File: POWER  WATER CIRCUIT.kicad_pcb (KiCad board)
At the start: 2 copper layers, 88.8 x 71.8 mm, 84 parts, among them IC1 DW01, J2 IN-, J3 IN+, J5 OUT +, J6 OUT -, Q1 FS8205A, Q2 BC817, Q3 IRLML5203, Q4 BC817, Q5 BC817, Q6 BC817, SW1 SW_MEC_5G, SW2 SW_MEC_5G, U1 LM2596S-ADJ, U2 TP4056, U3 LM1117MP-3.3, U4 ESP32-WROOM-32, U5 SIM800L-CORE, U6 MT3608

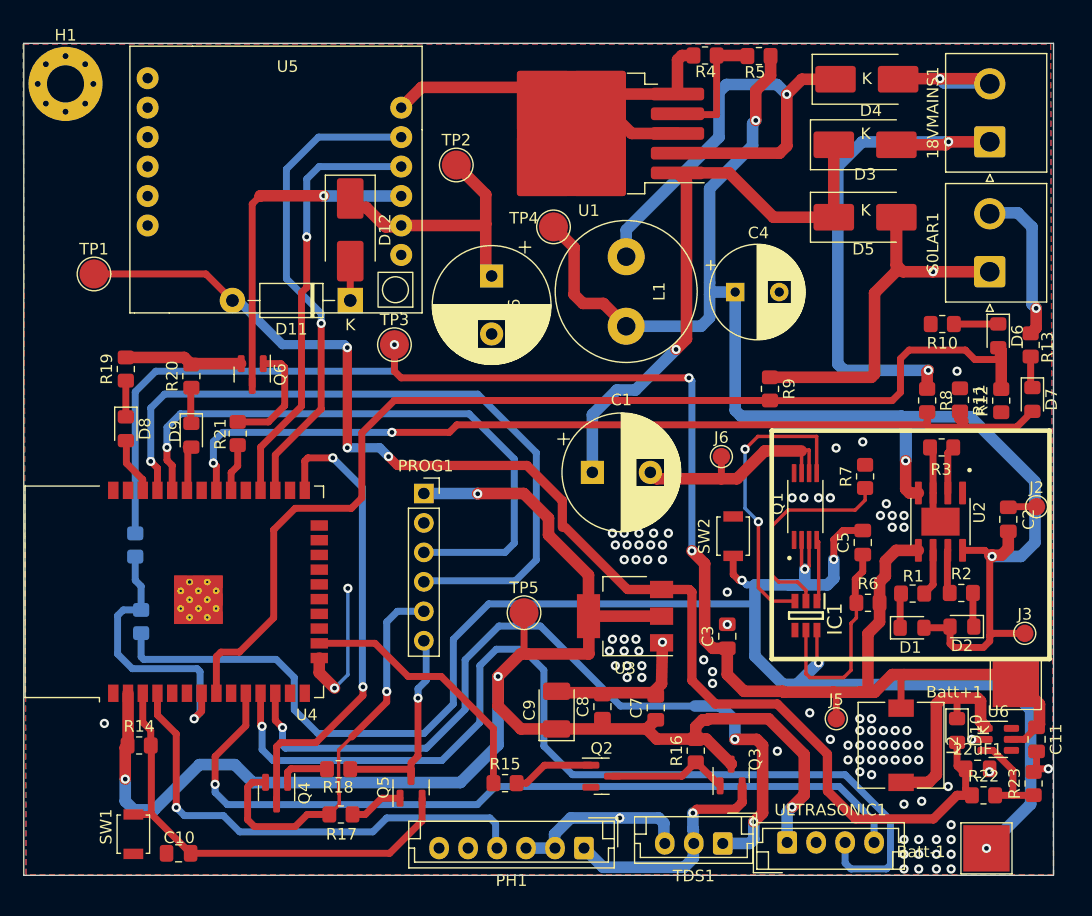
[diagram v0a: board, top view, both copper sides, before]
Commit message: Final Changes before production
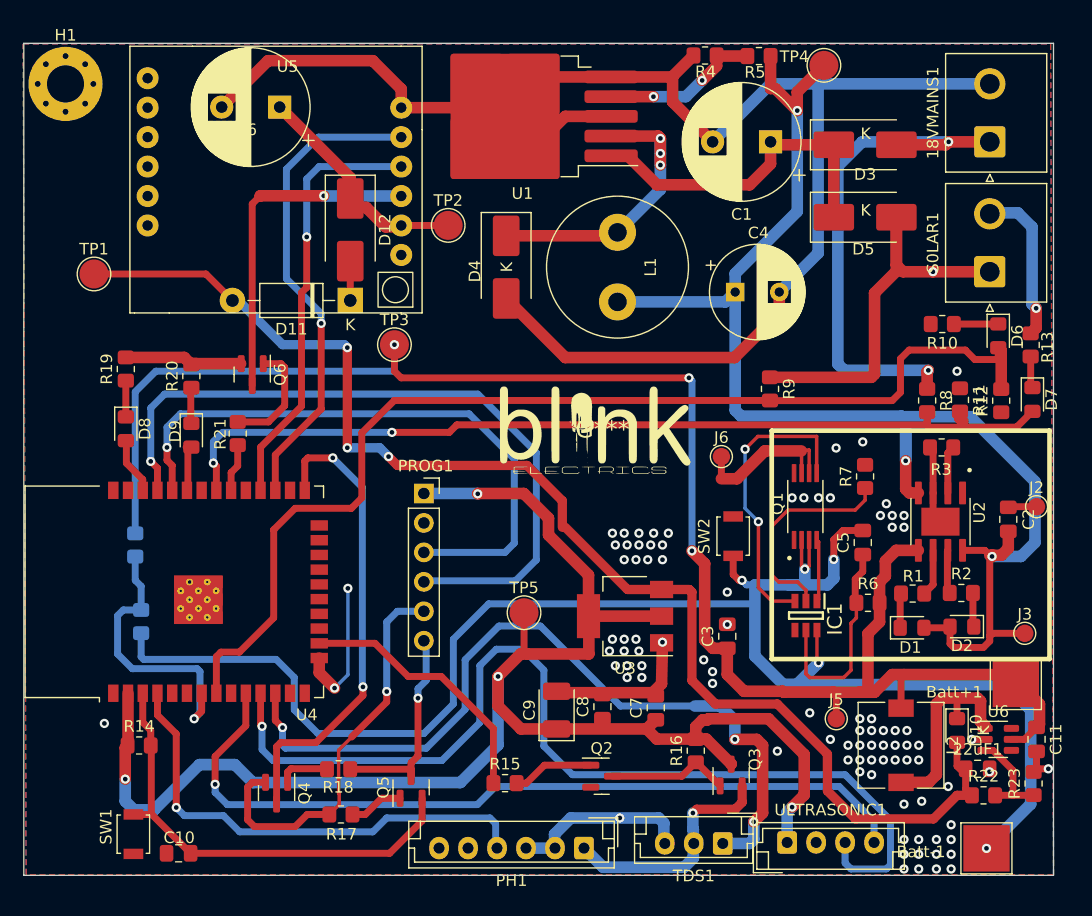
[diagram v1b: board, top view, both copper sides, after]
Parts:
- added G***: LOGO, blink logo:blink logo, F.Cu at (110.9, 89.1)
- moved D4 35.1 mm to (102.6, 75.1), turned to -90 degrees
- moved C1 32.4 mm to (125.4, 64.3), turned to 180 degrees
- moved TP4 27.2 mm to (130.0, 57.7)
- moved C6 23.4 mm to (83.1, 61.3), turned to 180 degrees
- moved U1 5.91 mm to (104.0, 62.1)
- moved TP2 5.25 mm to (97.6, 71.5)
- moved L1 2.23 mm to (112.2, 72.1)
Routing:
- net GND: track 145.7 -> 225.2 mm, vias 95 -> 94
- net + 18 V: track 51.8 -> 29.2 mm, vias 1 -> 0
- net Net-(D4-K): track 42.9 -> 26.0 mm, vias 1 -> 3
- net 6V: track 130.0 -> 122.3 mm
- net 4.0V: track 23.3 -> 19.6 mm
- net Net-(U1-FB): track 10.9 -> 13.8 mm, vias 0 -> 2
